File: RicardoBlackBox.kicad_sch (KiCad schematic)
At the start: 42 parts, among them J1 RBUS, U1 ESP32-S3, U5 LTC4411, Y1 40MHz±10ppm

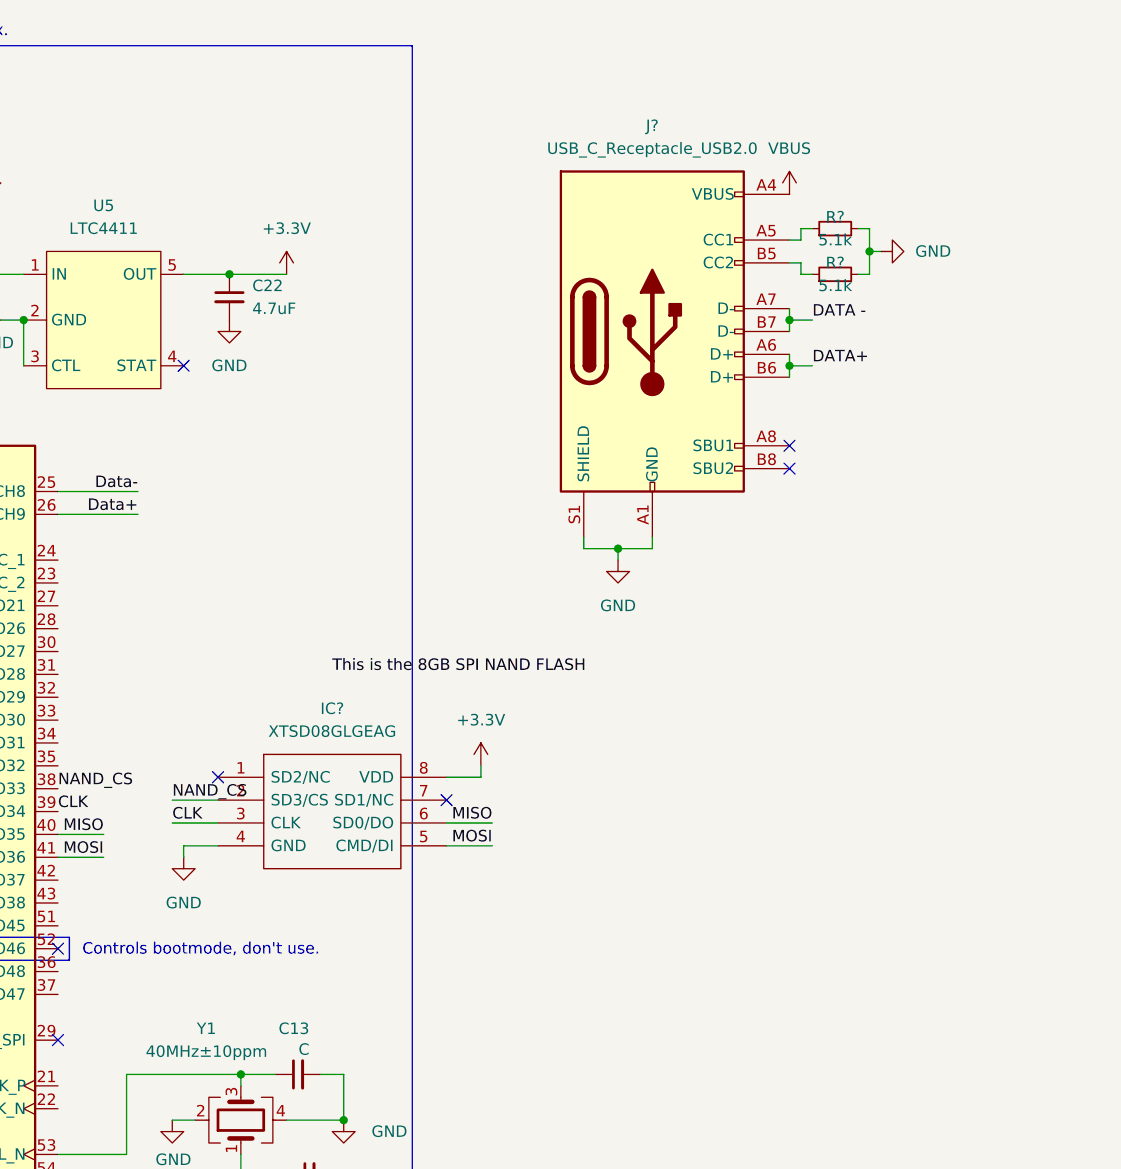
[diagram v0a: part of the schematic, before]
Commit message: PushingSecondSchematic
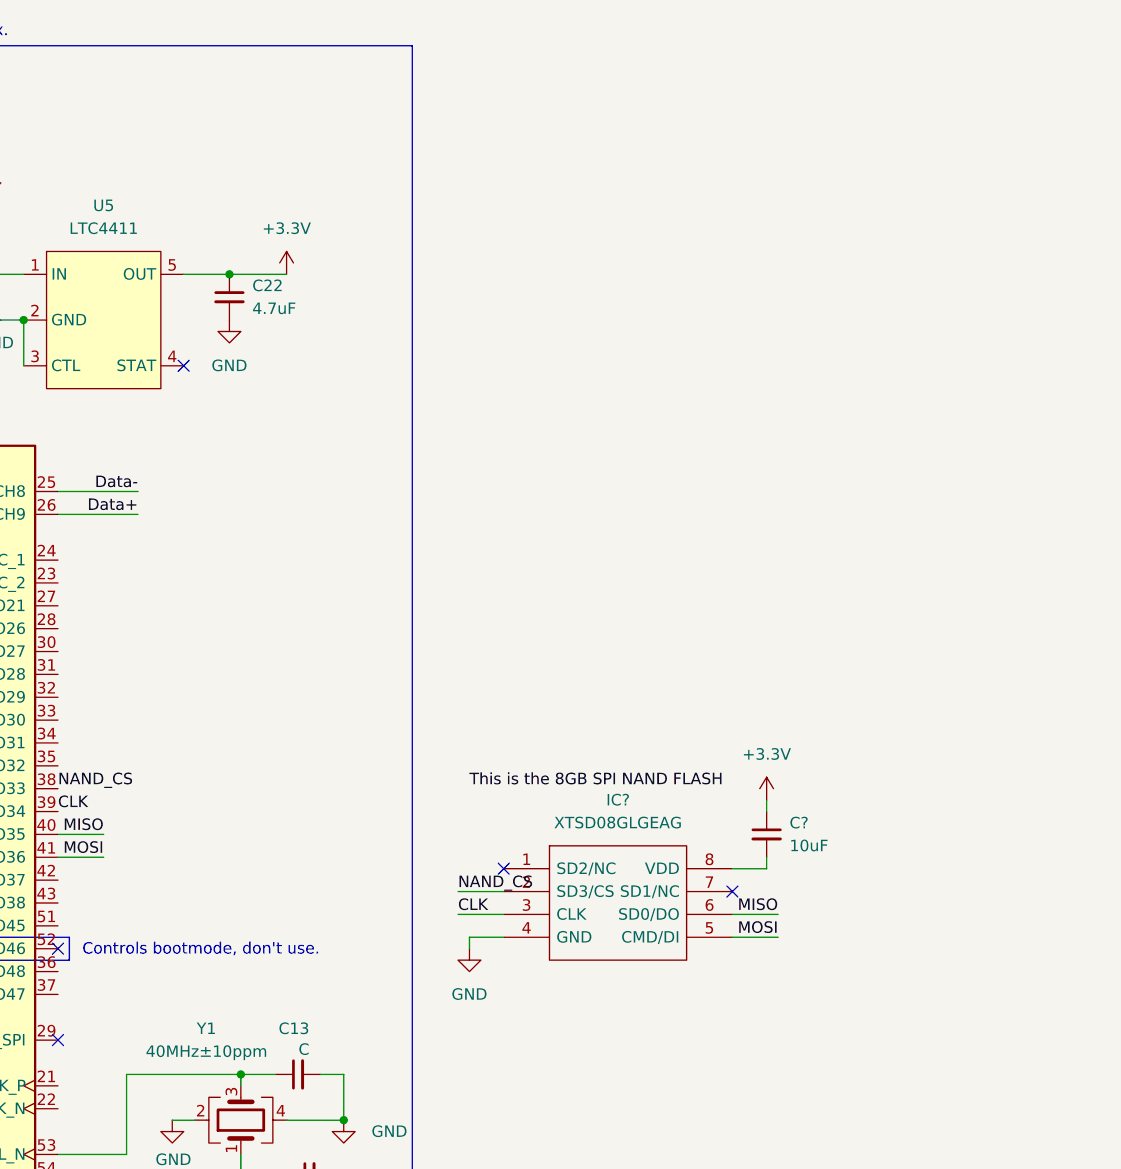
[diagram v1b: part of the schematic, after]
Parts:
- removed J?: USB_C_Receptacle_USB2.0, Connector_USB:USB_C_Receptacle_GCT_USB4085, symbol Connector:USB_C_Receptacle_USB2.0
- removed R? (x2): 5.1k, Resistor_SMD:R_0402_1005Metric, symbol Device:R_Small
- added C?: 10uF, symbol Device:C_Small
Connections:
- net +3V3: now also C?.1; no longer IC?.8 (VDD)
- new net: C?.2, IC?.8 (VDD)
- no-connect marks 8 -> 6
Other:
- moved on the sheet: IC?
